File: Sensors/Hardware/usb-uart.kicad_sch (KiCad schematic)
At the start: 16 parts, among them J15 USB_C_Receptacle_USB2.0, U10 SC4216H, U11 LTC4411

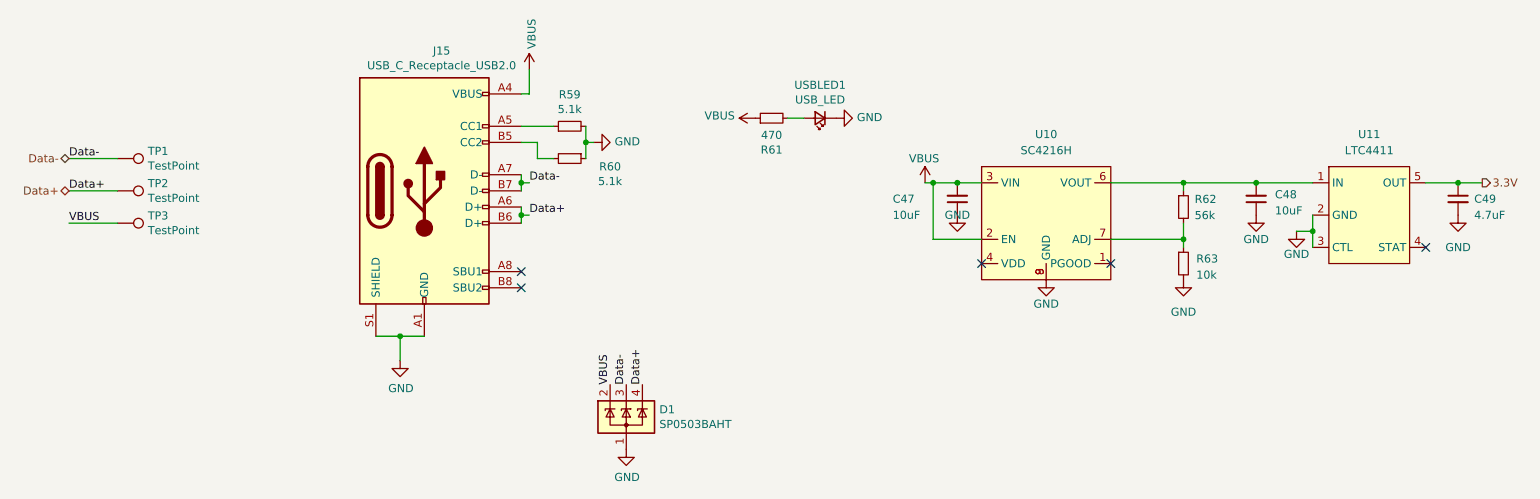
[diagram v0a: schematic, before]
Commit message: added 10V rail, moved to boosts sheet
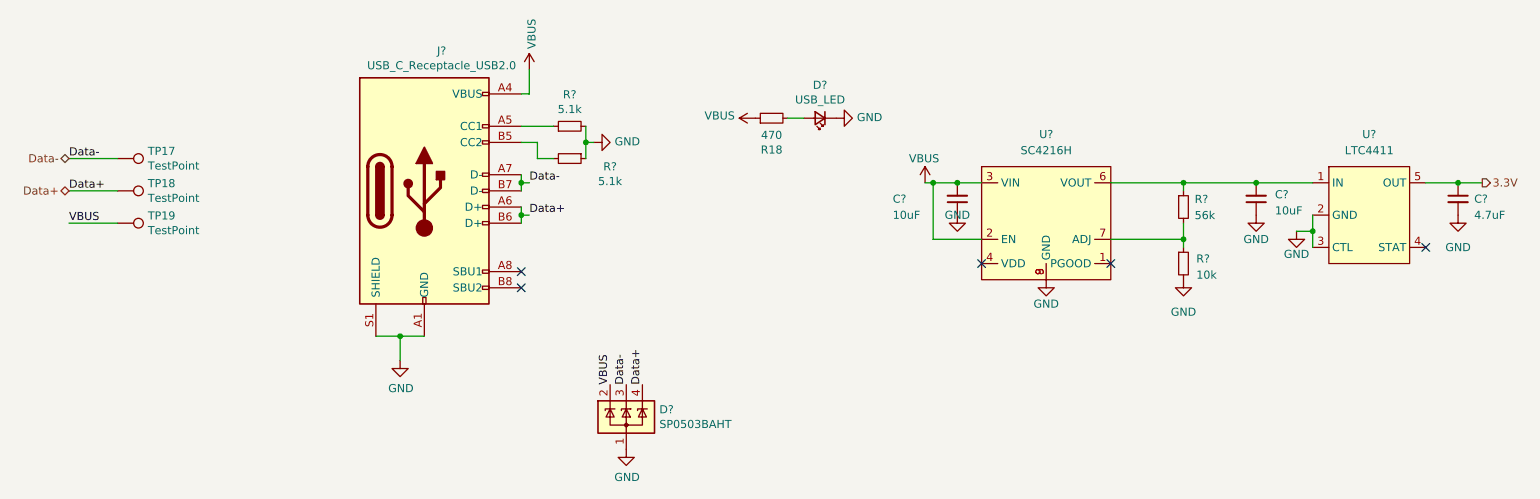
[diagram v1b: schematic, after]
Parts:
- renumbered C48 to C?, C47 to C?, C49 to C?, D1 to D?, USBLED1 to D?, J15 to J?, R61 to R18, R60 to R?, R59 to R?, R63 to R?, R62 to R?, TP1 to TP17, TP2 to TP18, TP3 to TP19, U11 to U?, U10 to U?
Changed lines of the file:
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@@
   (symbol (lib_id "power:GND") (at 127 96.52 90) (unit 1)
     (in_bom yes) (on_board yes)
-    (property "Reference" "#PWR0126" (id 0) (at 133.35 96.52 0)
+    (property "Reference" "#PWR?" (id 0) (at 133.35 96.52 0)
       (effects (font (size 1.27 1.27)) hide)
     )
@@
   (symbol (lib_id "Device:R_Small") (at 123.19 99.06 270) (unit 1)
     (in_bom yes) (on_board yes)
-    (property "Reference" "R60" (id 0) (at 129.54 100.33 90))
+    (property "Reference" "R?" (id 0) (at 129.54 100.33 90))
     (property "Value" "5.1k" (id 1) (at 129.54 102.6414 90))
     (property "Footprint" "Resistor_SMD:R_0402_1005Metric" (id 2) (at 123.19 99.06 0)
@@
   (symbol (lib_id "Device:R_Small") (at 123.19 93.98 90) (unit 1)
     (in_bom yes) (on_board yes)
-    (property "Reference" "R59" (id 0) (at 123.19 89.0016 90))
+    (property "Reference" "R?" (id 0) (at 123.19 89.0016 90))
     (property "Value" "5.1k" (id 1) (at 123.19 91.313 90))
     (property "Footprint" "Resistor_SMD:R_0402_1005Metric" (id 2) (at 123.19 93.98 0)
@@
   (symbol (lib_id "power:GND") (at 96.52 130.81 0) (unit 1)
     (in_bom yes) (on_board yes)
-    (property "Reference" "#PWR0124" (id 0) (at 96.52 137.16 0)
+    (property "Reference" "#PWR?" (id 0) (at 96.52 137.16 0)
       (effects (font (size 1.27 1.27)) hide)
     )
@@
   (symbol (lib_id "Connector:USB_C_Receptacle_USB2.0") (at 100.33 104.14 0) (unit 1)
     (in_bom yes) (on_board yes)
-    (property "Reference" "J15" (id 0) (at 103.0478 82.1182 0))
+    (property "Reference" "J?" (id 0) (at 103.0478 82.1182 0))
     (property "Value" "USB_C_Receptacle_USB2.0" (id 1) (at 103.0478 84.4296 0))
     (property "Footprint" "Connector_USB:USB_C_Receptacle_GCT_USB4085" (id 2) (at 104.14 104.14 0)
@@
   (symbol (lib_id "power:GND") (at 132.08 144.78 0) (unit 1)
     (in_bom yes) (on_board yes)
-    (property "Reference" "#PWR0127" (id 0) (at 132.08 151.13 0)
+    (property "Reference" "#PWR?" (id 0) (at 132.08 151.13 0)
       (effects (font (size 1.27 1.27)) hide)
     )
@@
   (symbol (lib_id "Power_Protection:SP0503BAHT") (at 132.08 139.7 0) (unit 1)
     (in_bom yes) (on_board yes)
-    (property "Reference" "D1" (id 0) (at 137.287 138.5316 0)
+    (property "Reference" "D?" (id 0) (at 137.287 138.5316 0)
       (effects (font (size 1.27 1.27)) (justify left))
     )
@@
   (symbol (lib_id "power:VBUS") (at 116.84 85.09 0) (unit 1)
     (in_bom yes) (on_board yes)
-    (property "Reference" "#PWR0125" (id 0) (at 116.84 88.9 0)
+    (property "Reference" "#PWR?" (id 0) (at 116.84 88.9 0)
       (effects (font (size 1.27 1.27)) hide)
     )
@@
   (symbol (lib_id "Connector:TestPoint") (at 52.07 99.06 270) (unit 1)
     (in_bom yes) (on_board yes)
-    (property "Reference" "TP1" (id 0) (at 56.8452 97.8916 90)
+    (property "Reference" "TP?" (id 0) (at 56.8452 97.8916 90)
       (effects (font (size 1.27 1.27)) (justify left))
     )
@@
   (symbol (lib_id "Connector:TestPoint") (at 52.07 104.14 270) (unit 1)
     (in_bom yes) (on_board yes)
-    (property "Reference" "TP2" (id 0) (at 56.8452 102.9716 90)
+    (property "Reference" "TP?" (id 0) (at 56.8452 102.9716 90)
       (effects (font (size 1.27 1.27)) (justify left))
     )
@@
   (symbol (lib_id "Connector:TestPoint") (at 52.07 109.22 270) (unit 1)
     (in_bom yes) (on_board yes)
-    (property "Reference" "TP3" (id 0) (at 56.8452 108.0516 90)
+    (property "Reference" "TP?" (id 0) (at 56.8452 108.0516 90)
       (effects (font (size 1.27 1.27)) (justify left))
     )
@@
   (symbol (lib_id "Device:LED_Small") (at 162.56 92.71 180) (unit 1)
     (in_bom yes) (on_board yes)
-    (property "Reference" "USBLED1" (id 0) (at 162.56 87.503 0))
+    (property "Reference" "USBLED?" (id 0) (at 162.56 87.503 0))
     (property "Value" "USB_LED" (id 1) (at 162.56 89.8144 0))
     (property "Footprint" "LED_SMD:LED_0603_1608Metric" (id 2) (at 162.56 92.71 90)
@@
   (symbol (lib_id "Device:R_Small") (at 154.94 92.71 90) (unit 1)
     (in_bom yes) (on_board yes)
-    (property "Reference" "R61" (id 0) (at 154.94 97.6884 90))
+    (property "Reference" "R?" (id 0) (at 154.94 97.6884 90))
     (property "Value" "470" (id 1) (at 154.94 95.377 90))
     (property "Footprint" "Resistor_SMD:R_0402_1005Metric" (id 2) (at 154.94 92.71 0)
@@
   (symbol (lib_id "power:GND") (at 165.1 92.71 90) (unit 1)
     (in_bom yes) (on_board yes)
-    (property "Reference" "#PWR0129" (id 0) (at 171.45 92.71 0)
+    (property "Reference" "#PWR?" (id 0) (at 171.45 92.71 0)
       (effects (font (size 1.27 1.27)) hide)
     )
@@
   (symbol (lib_id "power:VBUS") (at 152.4 92.71 90) (unit 1)
     (in_bom yes) (on_board yes)
-    (property "Reference" "#PWR0128" (id 0) (at 156.21 92.71 0)
+    (property "Reference" "#PWR?" (id 0) (at 156.21 92.71 0)
       (effects (font (size 1.27 1.27)) hide)
     )
@@
   (symbol (lib_id "iclr:LTC4411") (at 248.92 97.79 0) (unit 1)
     (in_bom yes) (on_board yes) (fields_autoplaced)
-    (property "Reference" "U11" (id 0) (at 248.92 95.25 0))
+    (property "Reference" "U?" (id 0) (at 248.92 95.25 0))
     (property "Value" "LTC4411" (id 1) (at 248.92 97.79 0))
     (property "Footprint" "Package_TO_SOT_SMD:SOT-23-5" (id 2) (at 248.92 97.79 0)
@@
   (symbol (lib_id "Device:C_Small") (at 231.14 105.41 180) (unit 1)
     (in_bom yes) (on_board yes)
-    (property "Reference" "C48" (id 0) (at 234.0983 104.7154 0)
+    (property "Reference" "C?" (id 0) (at 234.0983 104.7154 0)
       (effects (font (size 1.27 1.27)) (justify right))
     )
@@
   (symbol (lib_id "power:GND") (at 237.49 110.49 0) (unit 1)
     (in_bom yes) (on_board yes)
-    (property "Reference" "#PWR0135" (id 0) (at 237.49 116.84 0)
+    (property "Reference" "#PWR?" (id 0) (at 237.49 116.84 0)
       (effects (font (size 1.27 1.27)) hide)
     )
@@
   (symbol (lib_id "Device:R_Small") (at 219.71 115.57 0) (unit 1)
     (in_bom yes) (on_board yes)
-    (property "Reference" "R63" (id 0) (at 221.724 114.8197 0)
+    (property "Reference" "R?" (id 0) (at 221.724 114.8197 0)
       (effects (font (size 1.27 1.27)) (justify left))
     )
@@
   (symbol (lib_id "power:GND") (at 231.14 107.95 0) (unit 1)
     (in_bom yes) (on_board yes)
-    (property "Reference" "#PWR0134" (id 0) (at 231.14 114.3 0)
+    (property "Reference" "#PWR?" (id 0) (at 231.14 114.3 0)
       (effects (font (size 1.27 1.27)) hide)
     )
@@
   (symbol (lib_id "power:VBUS") (at 179.07 102.87 0) (unit 1)
     (in_bom yes) (on_board yes)
-    (property "Reference" "#PWR0130" (id 0) (at 179.07 106.68 0)
+    (property "Reference" "#PWR?" (id 0) (at 179.07 106.68 0)
       (effects (font (size 1.27 1.27)) hide)
     )
@@
   (symbol (lib_id "Device:R_Small") (at 219.71 106.68 0) (unit 1)
     (in_bom yes) (on_board yes)
-    (property "Reference" "R62" (id 0) (at 221.4667 105.4505 0)
+    (property "Reference" "R?" (id 0) (at 221.4667 105.4505 0)
       (effects (font (size 1.27 1.27)) (justify left))
     )
@@
   (symbol (lib_id "iclr:RT9025-25GSP") (at 198.12 101.6 0) (unit 1)
     (in_bom yes) (on_board yes) (fields_autoplaced)
-    (property "Reference" "U10" (id 0) (at 198.12 95.25 0))
+    (property "Reference" "U?" (id 0) (at 198.12 95.25 0))
     (property "Value" "SC4216H" (id 1) (at 198.12 97.79 0))
     (property "Footprint" "iclr:SOIC127P599X175-9N" (id 2) (at 198.12 96.52 0)
@@
   (symbol (lib_id "power:GND") (at 219.71 118.11 0) (unit 1)
     (in_bom yes) (on_board yes) (fields_autoplaced)
-    (property "Reference" "#PWR0133" (id 0) (at 219.71 124.46 0)
+    (property "Reference" "#PWR?" (id 0) (at 219.71 124.46 0)
       (effects (font (size 1.27 1.27)) hide)
     )
@@
   (symbol (lib_id "Device:C_Small") (at 184.15 105.41 180) (unit 1)
     (in_bom yes) (on_board yes)
-    (property "Reference" "C47" (id 0) (at 173.99 105.41 0)
+    (property "Reference" "C?" (id 0) (at 173.99 105.41 0)
       (effects (font (size 1.27 1.27)) (justify right))
     )
@@
   (symbol (lib_id "power:GND") (at 262.89 107.95 0) (unit 1)
     (in_bom yes) (on_board yes) (fields_autoplaced)
-    (property "Reference" "#PWR0136" (id 0) (at 262.89 114.3 0)
+    (property "Reference" "#PWR?" (id 0) (at 262.89 114.3 0)
       (effects (font (size 1.27 1.27)) hide)
     )
@@
   (symbol (lib_id "power:GND") (at 198.12 118.11 0) (unit 1)
     (in_bom yes) (on_board yes)
-    (property "Reference" "#PWR0132" (id 0) (at 198.12 124.46 0)
+    (property "Reference" "#PWR?" (id 0) (at 198.12 124.46 0)
       (effects (font (size 1.27 1.27)) hide)
     )
@@
   (symbol (lib_id "Device:C_Small") (at 262.89 105.41 0) (unit 1)
     (in_bom yes) (on_board yes)
-    (property "Reference" "C49" (id 0) (at 265.43 105.41 0)
+    (property "Reference" "C?" (id 0) (at 265.43 105.41 0)
       (effects (font (size 1.27 1.27)) (justify left))
     )
@@
   (symbol (lib_id "power:GND") (at 184.15 107.95 0) (unit 1)
     (in_bom yes) (on_board yes)
-    (property "Reference" "#PWR0131" (id 0) (at 184.15 114.3 0)
-      (effects (font (size 1.27 1.27)) hide)
-    )
+    (property "Reference" "#PWR?" (id 0) (at 184.15 114.3 0)
+      (effects (font (size 1.27 1.27)) hide)
+    )
